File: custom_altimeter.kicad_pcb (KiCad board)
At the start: 2 copper layers, 4 parts, among them U1 FEATHERWING_NODIM

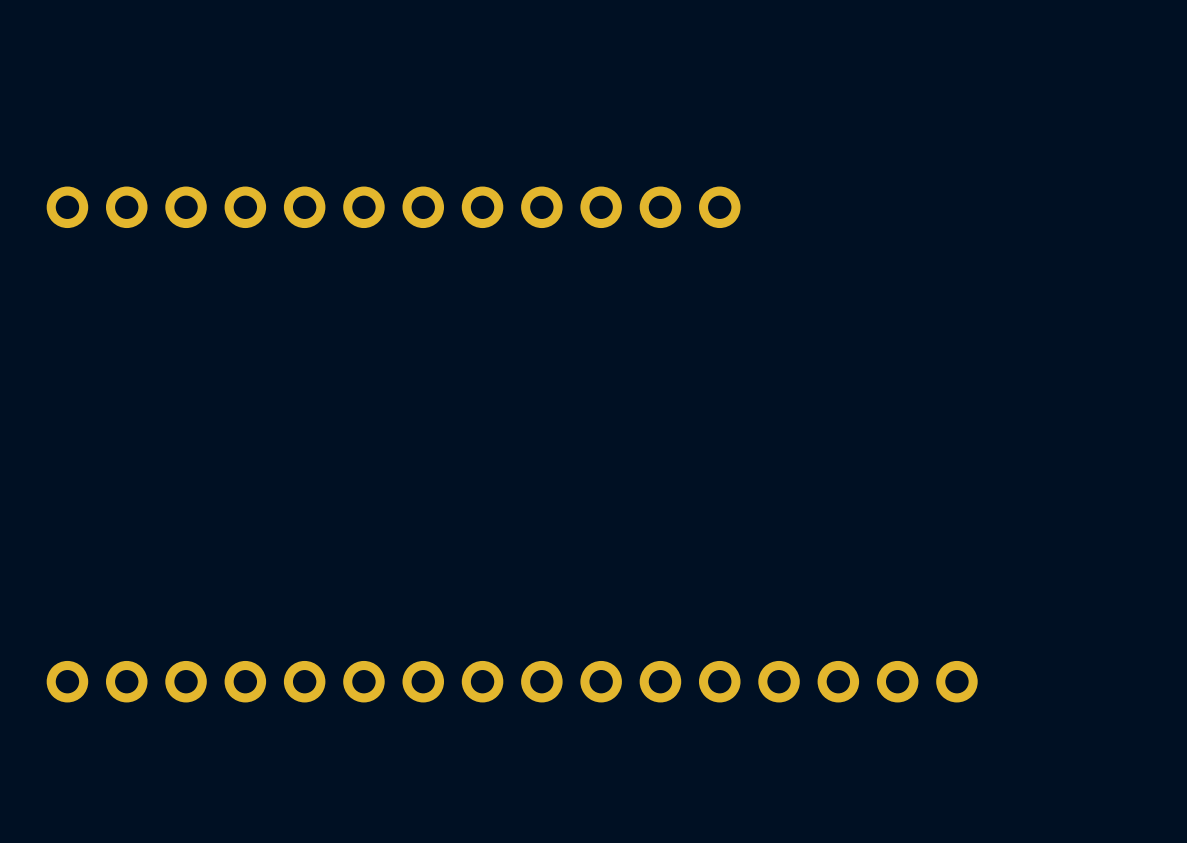
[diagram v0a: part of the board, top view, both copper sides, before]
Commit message: Additional fixes
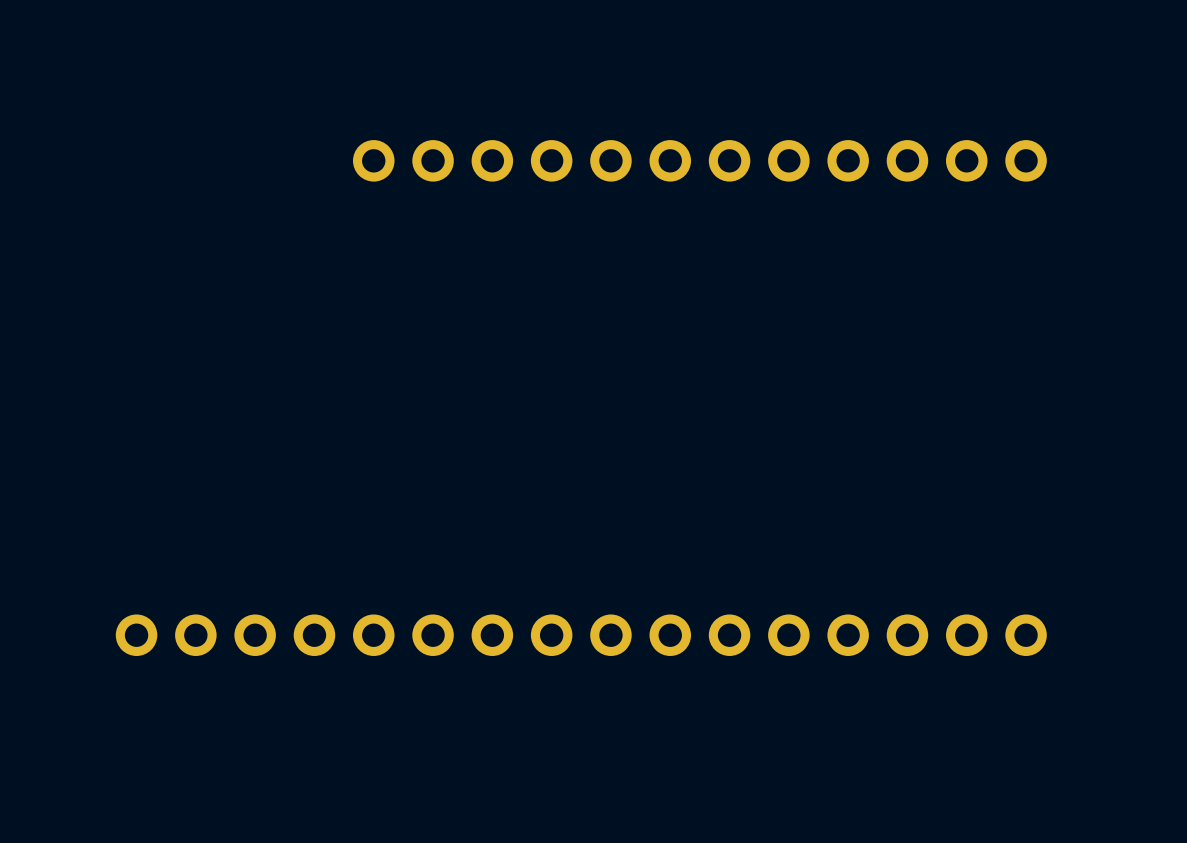
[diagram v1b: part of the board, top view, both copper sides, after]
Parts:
- U1: moved to F.Cu
- moved U1 47.9 mm to (48.7, 127.3), turned to 0 degrees
